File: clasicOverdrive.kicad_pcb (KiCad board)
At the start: 2 copper layers, 50.8 x 80 mm, 43 parts, among them CON1 SN49B12B, CON2 SN49B12B, J1 Jack-DC, Q1 2N2222, Q2 2N2222, U1 foot_switch, U2 LM4562

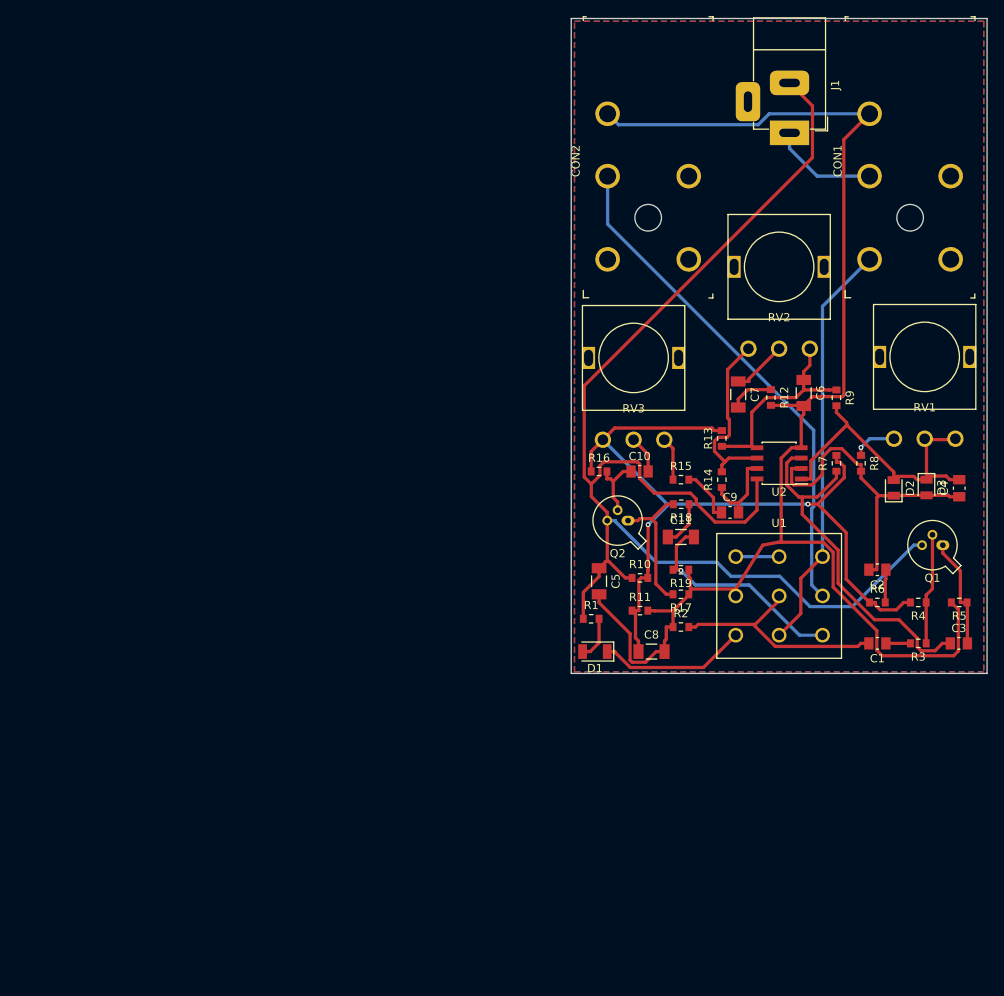
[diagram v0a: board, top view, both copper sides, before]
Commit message: Board Finished
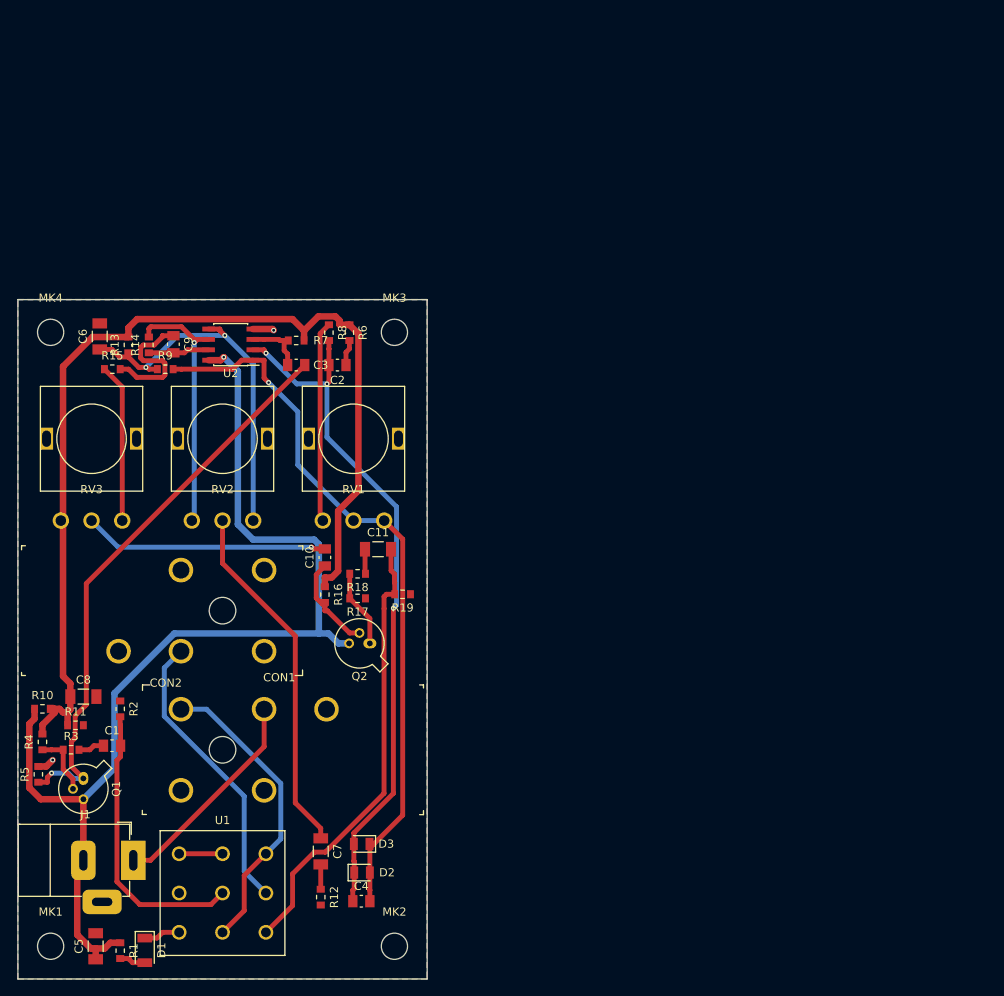
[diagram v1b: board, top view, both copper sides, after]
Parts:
- added MK1: Mounting_Hole, MountingHole:MountingHole_3.2mm_M3, F.Cu at (104.0, 146.2)
- added MK2: Mounting_Hole, MountingHole:MountingHole_3.2mm_M3, F.Cu at (146.0, 146.2)
- added MK3: Mounting_Hole, MountingHole:MountingHole_3.2mm_M3, F.Cu at (146.0, 71.2)
- added MK4: Mounting_Hole, MountingHole:MountingHole_3.2mm_M3, F.Cu at (104.0, 71.2)
- moved J1 119.7 mm to (114.1, 135.7), turned to 0 degrees
- moved R5 114.4 mm to (102.5, 125.2), turned to 90 degrees
- moved Q1 108.8 mm to (108.0, 125.7), turned to 270 degrees
- moved R4 108.3 mm to (103.0, 121.3), turned to 90 degrees
- moved CON1 106.2 mm to (125.0, 122.2), turned to 0 degrees
- moved R3 104.3 mm to (106.5, 122.2), turned to 0 degrees
- moved C1 94.3 mm to (111.5, 121.7), turned to 0 degrees
- moved C4 88.8 mm to (142.0, 140.7), turned to 0 degrees
- moved C3 87.8 mm to (134.0, 75.2)
- moved C6 86.3 mm to (110.0, 71.7), turned to 90 degrees
- moved R12 82.2 mm to (137.0, 140.2)
- moved R9 82.1 mm to (118.0, 75.7), turned to 0 degrees
- moved D3 81.6 mm to (142.0, 133.7), turned to 180 degrees
- moved D2 80.2 mm to (142.1, 137.2), turned to 0 degrees
- moved U1 77.1 mm to (125.0, 139.7)
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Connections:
- RV1 pad 4: (no net) -> GND
- RV1 pad 5: (no net) -> GND
- RV2 pad 4: (no net) -> GND
- RV2 pad 5: (no net) -> GND
- RV3 pad 4: (no net) -> GND
- RV3 pad 5: (no net) -> GND
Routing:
- net GND: track 179.1 -> 4.69 mm, vias 0 -> 2
- net Net-(C3-Pad2): track 13.9 -> 69.5 mm, vias 0 -> 1
- net Net-(C4-Pad2): track 38.6 -> 89.1 mm, vias 0 -> 1
- net Net-(C2-Pad2): track 40.1 -> 85.3 mm, vias 0 -> 3
- net Net-(C7-Pad1): track 6.83 -> 43.8 mm
- net Net-(C3-Pad1): track 43.7 -> 7.57 mm
- net +9V: track 161.4 -> 133.1 mm, vias 0 -> 1
- net +4V5: track 98.6 -> 126.5 mm, vias 2 -> 0
- net Net-(C11-Pad2): track 27.1 -> 54.9 mm, vias 1 -> 0
- net Net-(CON2-PadR): track 62.4 -> 35.5 mm
- net Net-(C10-Pad2): track 4.61 -> 29.9 mm, vias 0 -> 1
- net Net-(C6-Pad1): track 25.4 -> 46.3 mm, vias 0 -> 2
- net Net-(R8-Pad1): track 5.44 -> 24.5 mm, vias 1 -> 0
- net Net-(R15-Pad1): track 5.32 -> 19.4 mm
- net Net-(D1-Pad1): track 18.2 -> 4.49 mm
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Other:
- board size 50.8 x 80 mm -> 50 x 83 mm
- net class Default: trace_width 0.4 -> 0.6
- net class PWR added: clearance 0.2, trace_width 0.8, via_dia 0.6, via_drill 0.35
